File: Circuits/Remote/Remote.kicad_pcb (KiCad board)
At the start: 2 copper layers, 80 x 68.1 mm, 31 parts, among them CN1 WRITER, Q1 2SK4017, SW1 WakeUp, U1 TWE_LITE_DIP, U2 STEPUPDIP3.3V, U3 ATP3011-PU, U4 HT82V739

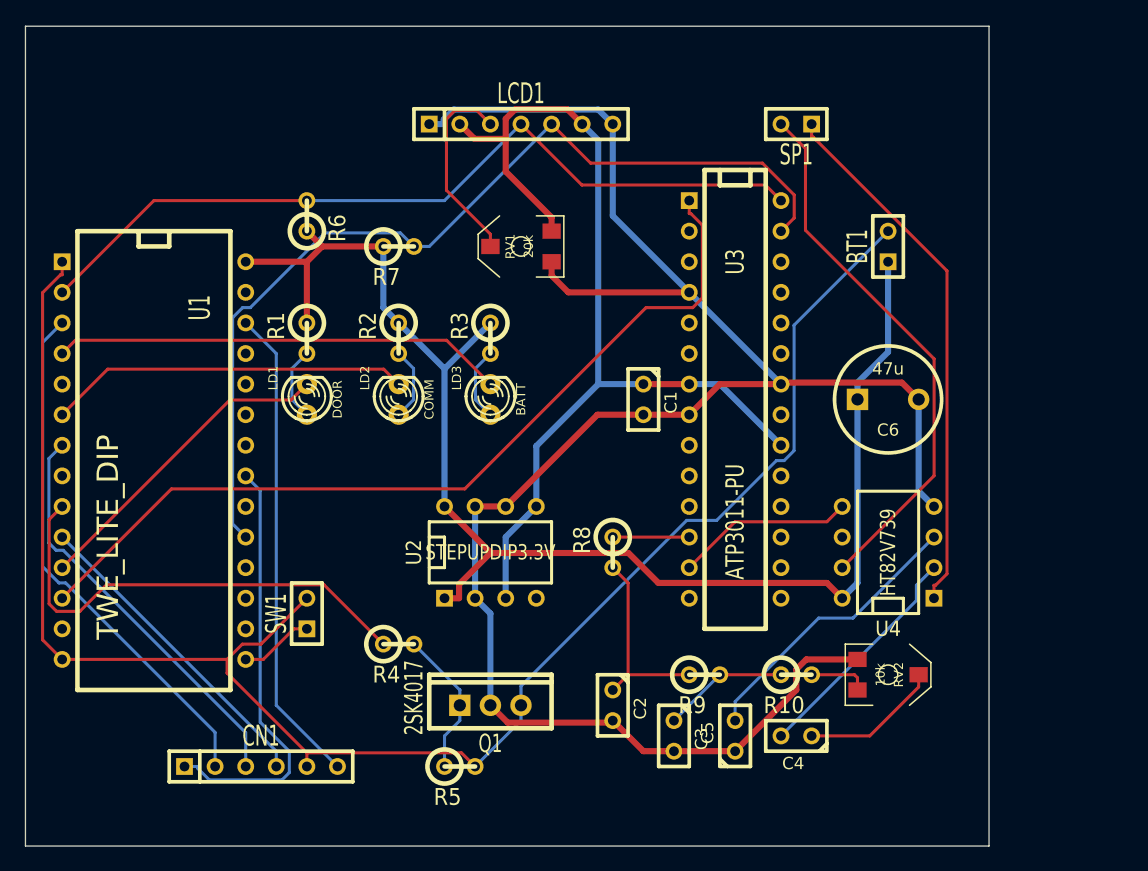
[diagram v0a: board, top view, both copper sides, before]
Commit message: Consider NTH.
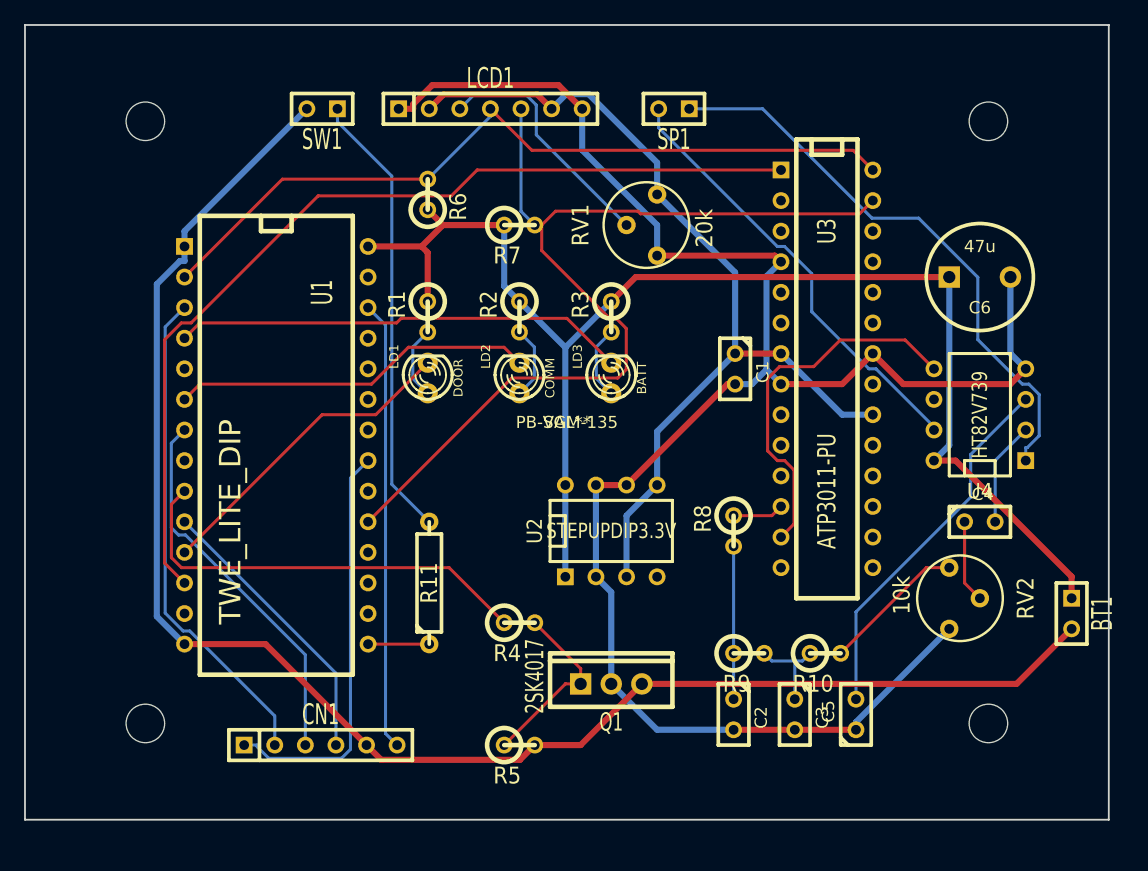
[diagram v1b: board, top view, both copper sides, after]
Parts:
- added PB-SGM-135: VAL**, PB-SGM-135, F.Cu at (57.1, 45.1)
- added R11: 10k, R4, F.Cu at (45.7, 58.4)
- RV1, RV2: footprint POT_CMS -> RV2
- moved SW1 41.9 mm to (36.8, 19.1), turned to 180 degrees
- moved BT1 34.1 mm to (99.1, 61.0), turned to 270 degrees
- moved C4 23.4 mm to (91.4, 53.3), turned to 0 degrees
- moved U4 13.7 mm to (91.4, 44.5)
- moved C6 12.7 mm to (91.4, 33.0)
- moved U1 10.2 mm to (33.0, 47.0)
- moved SP1 10.2 mm to (66.0, 19.1)
- moved C5 10.2 mm to (81.2, 69.3)
- moved LD1 10.2 mm to (45.6, 41.4)
- moved LD2 10.2 mm to (53.2, 41.4)
- moved LD3 10.2 mm to (60.8, 41.4)
- moved R1 10.2 mm to (45.6, 36.3)
- moved R2 10.2 mm to (53.2, 36.3)
- moved R3 10.2 mm to (60.8, 36.3)
- moved R4 10.2 mm to (53.2, 61.7)
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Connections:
- net N-000001 renamed /V0
- net N-0000021 renamed /LPF2
- net N-0000022 renamed /LPF1
- net N-0000023 renamed /AOUT
- net N-0000025 renamed /VOL
- net N-0000027 renamed /PLAY#
- net N-0000029 renamed /VREF
- net N-000003 renamed /PWM4
- net N-0000030 renamed /AudioIn
- net N-0000031 renamed /PWM2
- net N-000004 renamed /3V_Gate
- net N-000005 renamed /LD1
- net N-0000050 renamed /PWM1
- net N-000006 renamed /LD2
- net N-000007 renamed /LD3
- net N-000009 renamed /G
- R10 pad 2: N-0000020 -> /LPF3
- RV2 pad 1: /QGND -> /LPF3
- RV2 pad 3: N-0000020 -> /QGND
- SW1 pad 1: /WUP -> N-0000016
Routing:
- net N-0000016: track 0.00 -> 37.4 mm
- net /PLAY#: track 14.8 -> 31.0 mm
- net /LPF3: track 0.00 -> 12.0 mm
- net /AudioIn: track 19.2 -> 8.67 mm
- net GND: track 143.4 -> 132.9 mm
- net /SPK-: track 45.3 -> 36.8 mm
- net /QGND: track 161.5 -> 153.3 mm
- net /VREF: track 23.7 -> 30.7 mm
- net /RESET#: track 72.1 -> 77.9 mm
- net /3.3V: track 82.8 -> 77.1 mm
- net N-0000020: track 4.93 -> 0.00 mm
- net /VOL: track 11.6 -> 6.88 mm
- net /V0: track 16.5 -> 20.2 mm
- net /3V_Gate: track 39.5 -> 35.8 mm
- net /LPF1: track 16.3 -> 12.7 mm
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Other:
- board size 80 x 68.1 mm -> 90 x 66 mm
